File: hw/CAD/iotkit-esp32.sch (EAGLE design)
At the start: 4 parts

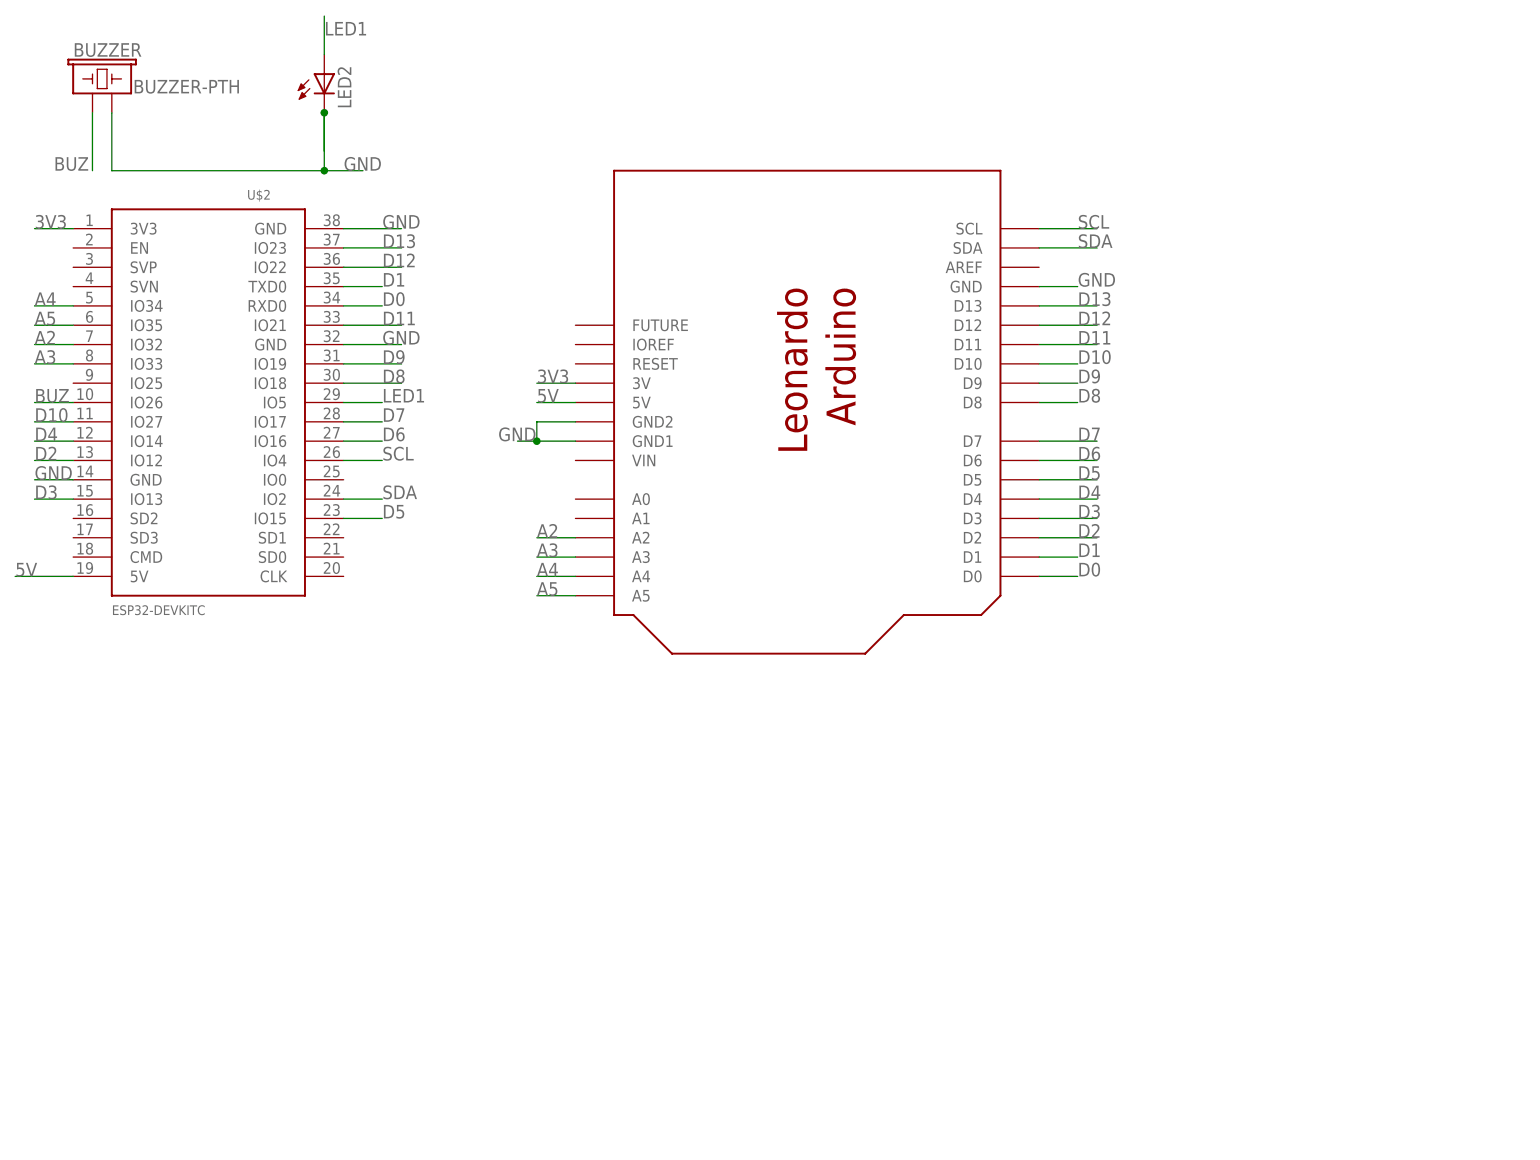
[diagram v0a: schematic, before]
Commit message: Inkl. Stepper
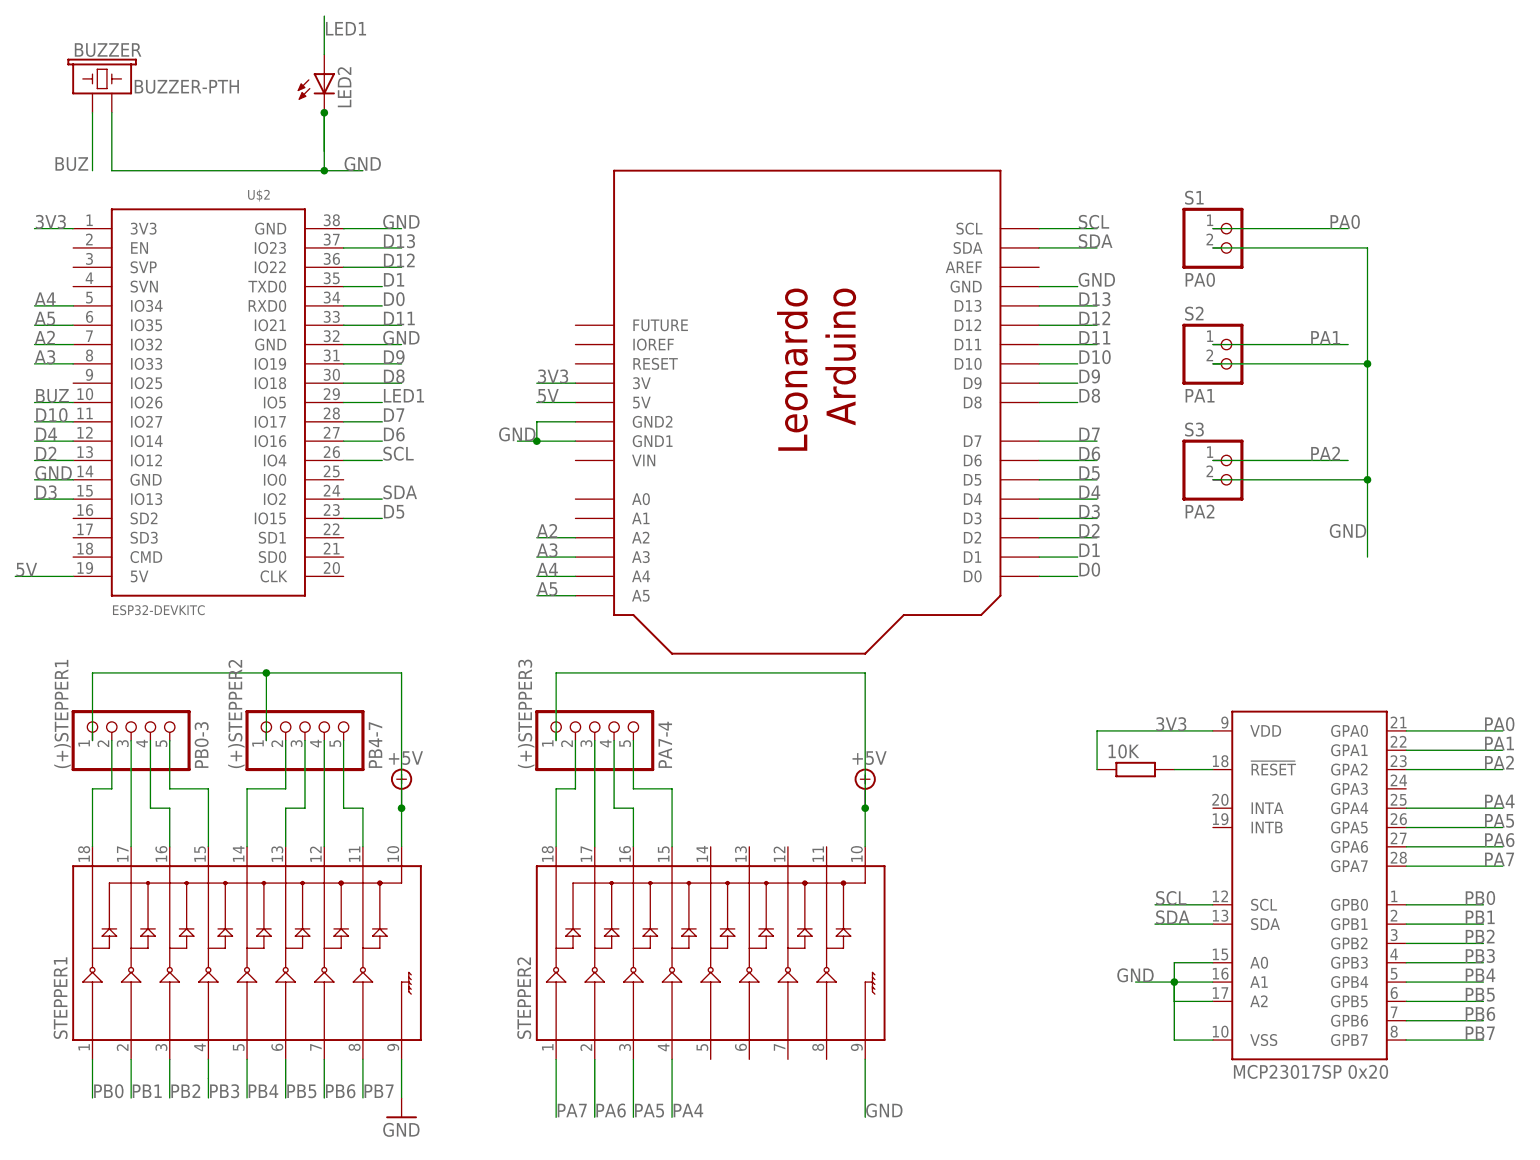
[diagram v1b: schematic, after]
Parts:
- added (+)STEPPER1: PB0-3, pinhead:PINHD-1X5
- added (+)STEPPER2: PB4-7, pinhead:PINHD-1X5
- added (+)STEPPER3: PA7-4, pinhead:PINHD-1X5
- added 10K: (no value), rcl:R-EU_0204/7
- added IC1: MCP23017SP 0x20, microchip:MCP23017SP
- added S1: PA0, pinhead:PINHD-1X2
- added S2: PA1, pinhead:PINHD-1X2
- added S3: PA2, pinhead:PINHD-1X2
- added STEPPER1, STEPPER2: (no value), SparkFun-IC-Special-Function:ULN2803DIP
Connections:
- new net +5V: (+)STEPPER1.1, (+)STEPPER2.1, (+)STEPPER3.1, STEPPER1.10, STEPPER2.10
- new net N$1: (+)STEPPER2.2, STEPPER1.14
- new net N$2: (+)STEPPER2.3, STEPPER1.13
- new net N$3: (+)STEPPER2.4, STEPPER1.12
- new net N$30: (+)STEPPER1.2, STEPPER1.18
- new net N$31: (+)STEPPER1.3, STEPPER1.17
- new net N$32: (+)STEPPER1.4, STEPPER1.16
- new net N$33: (+)STEPPER1.5, STEPPER1.15
- new net N$4: (+)STEPPER2.5, STEPPER1.11
- new net N$5: 10K.2, IC1.!RESET
- new net N$6: (+)STEPPER3.2, STEPPER2.18
- new net N$7: (+)STEPPER3.3, STEPPER2.17
- new net N$8: (+)STEPPER3.4, STEPPER2.16
- new net N$9: (+)STEPPER3.5, STEPPER2.15
- new net PA0: IC1.GPA0, S1.1
- new net PA1: IC1.GPA1, S2.1
- new net PA2: IC1.GPA2, S3.1
- new net PA4: IC1.GPA4, STEPPER2.4
- new net PA5: IC1.GPA5, STEPPER2.3
- new net PA6: IC1.GPA6, STEPPER2.2
- new net PA7: IC1.GPA7, STEPPER2.1
- new net PB0: IC1.GPB0, STEPPER1.1
- new net PB1: IC1.GPB1, STEPPER1.2
- new net PB2: IC1.GPB2, STEPPER1.3
- new net PB3: IC1.GPB3, STEPPER1.4
- new net PB4: IC1.GPB4, STEPPER1.5
- new net PB5: IC1.GPB5, STEPPER1.6
- new net PB6: IC1.GPB6, STEPPER1.7
- new net PB7: IC1.GPB7, STEPPER1.8
- net 3V3: now also 10K.1, IC1.VDD
- net GND: now also IC1.A0, IC1.A1, IC1.A2, IC1.VSS, S1.2, S2.2, S3.2, STEPPER1.9, STEPPER2.9
- net SCL: now also IC1.SCL
- net SDA: now also IC1.SDA
